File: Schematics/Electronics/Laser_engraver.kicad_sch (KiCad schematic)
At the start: 9 parts, among them J2 MOT_X_SOCK_1, J3 MOT_Y_SOCK, J4 Power, J5 FinalSock, U5 LM7805_TO220

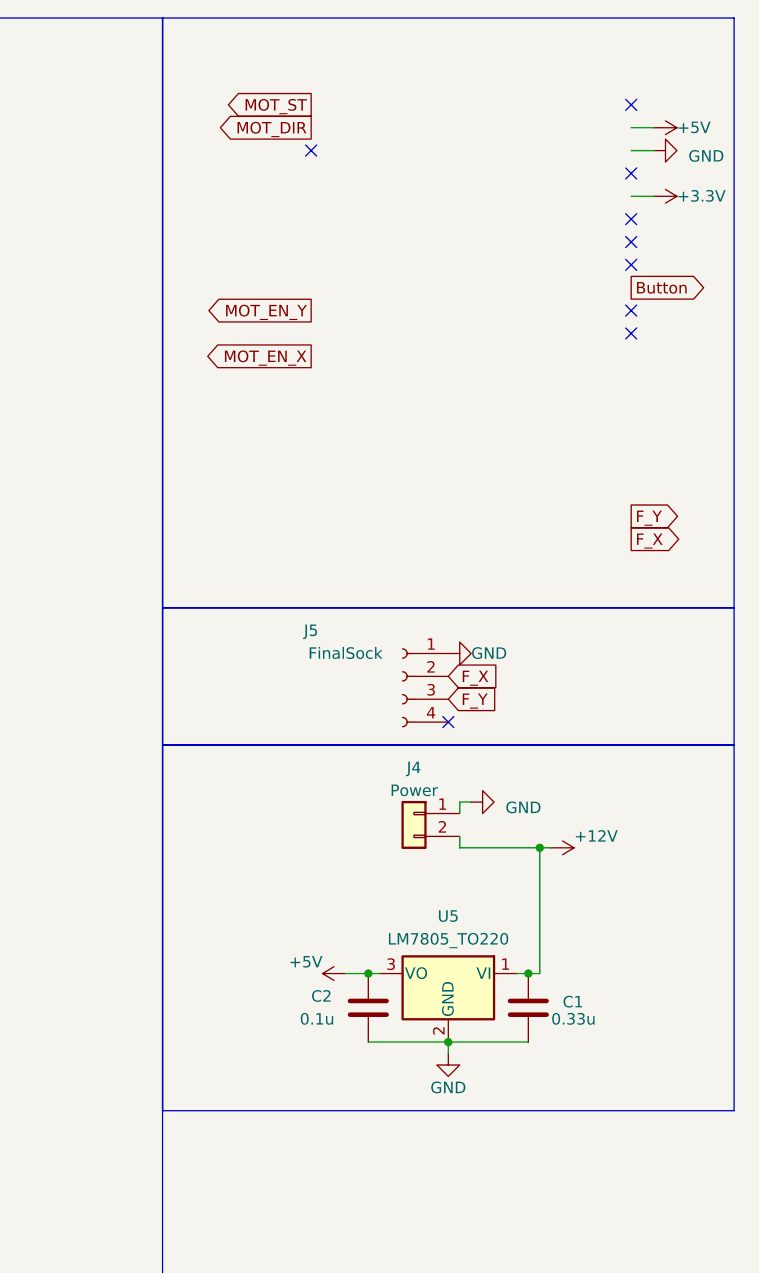
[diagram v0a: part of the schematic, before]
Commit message: Modifying schematics
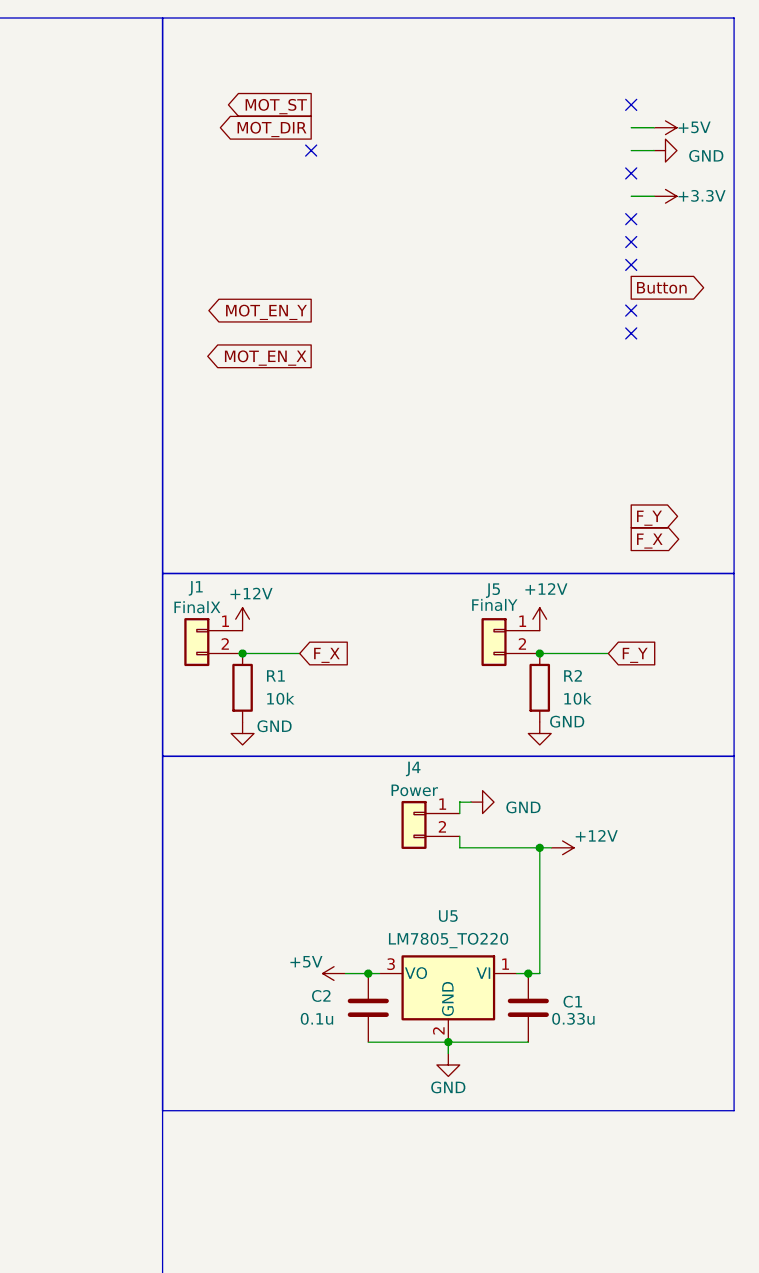
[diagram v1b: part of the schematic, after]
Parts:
- removed J5: FinalSock, Connector_PinSocket_2.54mm:PinSocket_1x04_P2.54mm_Vertical, symbol Connector:Conn_01x04_Socket
- added J1: FinalX, symbol Connector_Generic:Conn_01x02
- added J5: FinalY, symbol Connector_Generic:Conn_01x02
- added R1, R2: 10k, symbol Device:R
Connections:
- net +12V: now also J1.1 (Pin_1), J5.1 (Pin_1)
- net F_X: now also J1.2 (Pin_2), R1.1
- net F_Y: now also J5.2 (Pin_2), R2.1
- net GND: now also R1.2, R2.2
- no-connect marks 15 -> 14
